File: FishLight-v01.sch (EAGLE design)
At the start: 214 parts, among them Q1 RK7002BSOT23-3, Q10 RK7002BSOT23-3, Q11 RK7002BSOT23-3, Q12 RK7002BSOT23-3, Q13 RK7002BSOT23-3, Q14 RK7002BSOT23-3, Q15 RK7002BSOT23-3, Q2 RK7002BSOT23-3, Q3 RK7002BSOT23-3, Q4 RK7002BSOT23-3, Q5 RK7002BSOT23-3, Q6 RK7002BSOT23-3, Q7 RK7002BSOT23-3, Q8 RK7002BSOT23-3, Q9 RK7002BSOT23-3, U1 SPARK_CORECORE, U10 AD5248MSOP-10, U11 INA219SOT23-8, U12 INA219SOT23-8, U13 INA219SOT23-8, U14 INA219SOT23-8, U15 INA219SOT23-8, U16 MIC29300D2PAK-3, U17 L7805D2PAK-2, U2 DS3231MSOIC-8, U22 AD5248MSOP-10, U23 CAT4101TO-263, U24 CAT4101TO-263, U25 CAT4101TO-263, U26 INA219SOT23-8, U27 INA219SOT23-8, U28 INA219SOT23-8, U29 CD74HC4067SSOP24, U3 CAT4101TO-263, U30 CD74HC4067SSOP24, U31 RELAY-SOLIDSTATEPTH, U32 RELAY-SOLIDSTATEPTH, U33 RELAY-SOLIDSTATEPTH, U34 NC7SZ373TSSOP-6, U35 NC7SZ373TSSOP-6, U36 NC7SZ373TSSOP-6, U37 NC7SZ373TSSOP-6, U38 NC7SZ373TSSOP-6, U39 NC7SZ373TSSOP-6, U4 CAT4101TO-263, U40 NC7SZ373TSSOP-6, U41 NC7SZ373TSSOP-6, U42 NC7SZ373TSSOP-6, U43 NC7SZ373TSSOP-6, U44 NC7SZ373TSSOP-6, U45 NC7SZ373TSSOP-6, U46 NC7SZ373TSSOP-6, U47 NC7SZ373TSSOP-6, U48 NC7SZ373TSSOP-6, U5 CAT4101TO-263, U6 CAT4101TO-263, U7 CAT4101TO-263, U8 AD5248MSOP-10, U9 AD5248MSOP-10

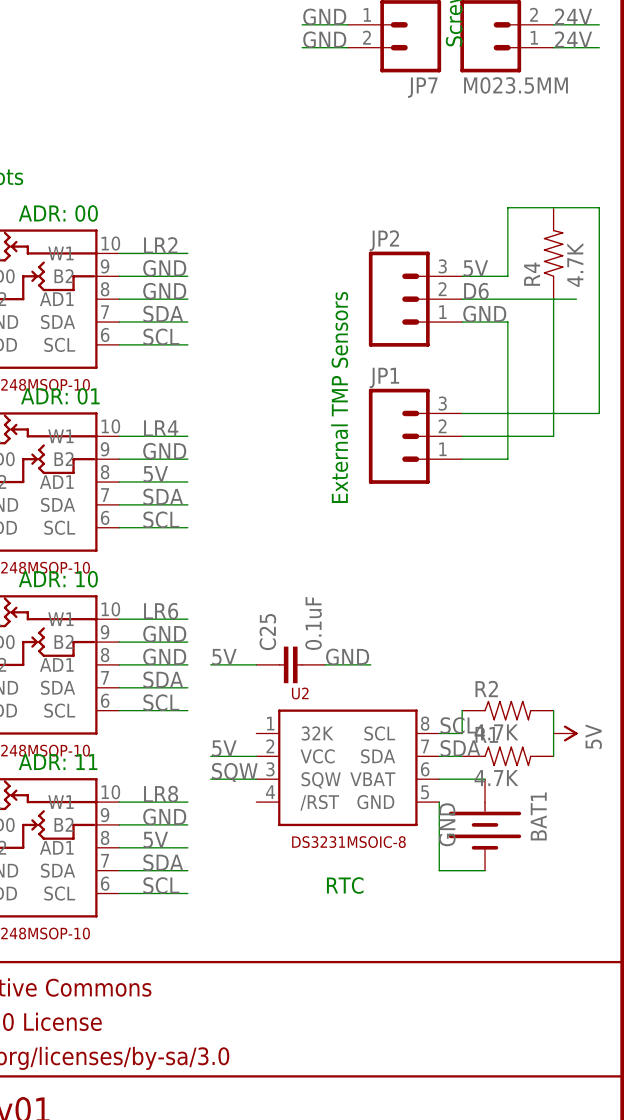
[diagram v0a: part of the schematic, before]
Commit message: FishLight_PCB: Routed power lines and sized them right
Moved a few things around and then routed the power lines for the
12V and 24V lines.  Also sized them appropriately for their max
current of about 7A and 15A respectively.
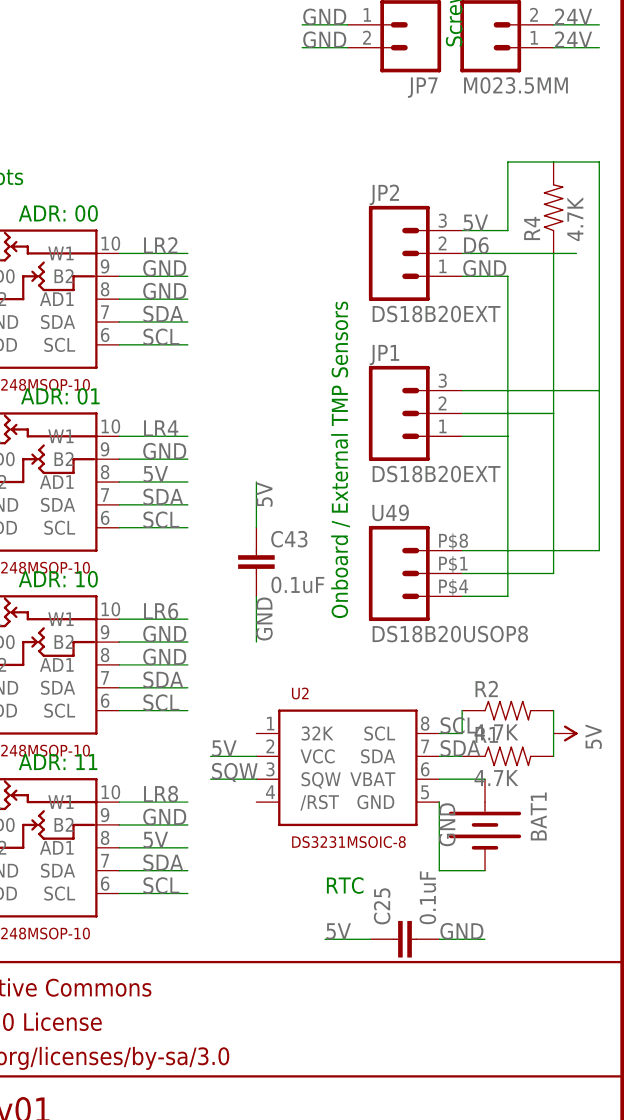
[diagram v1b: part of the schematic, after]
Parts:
- added C43: 0.1uF, SparkFun-Capacitors:0.1UF-25V(+80/-20%)(0603)
- added U49: DS18B20USOP8, Mikes-Stuff:DS18B20USOP8
- JP1, JP2: value (none) -> DS18B20EXT; device Mikes-Stuff:M03POLAR -> Mikes-Stuff:DS18B20EXT
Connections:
- net 5V: now also C43.1, JP1.VDD, JP2.VDD, U49.VDD; no longer JP1.3, JP2.3
- net D6: now also JP1.DQ, JP2.DQ, U49.DQ; no longer JP1.2, JP2.2
- net GND: now also C43.2, JP1.GND, JP2.GND, U49.GND; no longer JP1.1, JP2.1
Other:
- note added: "Onboard / External TMP Sensors"
- note removed: "External TMP Sensors"
- moved on the sheet: C25, JP1, JP2, R4
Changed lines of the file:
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@@
 <part name="C6" library="SparkFun-Capacitors" deviceset="0.1UF-100V-10%(0603)" device="" value="0.1uF"/>
 <part name="C12" library="SparkFun-Capacitors" deviceset="CAP" device="0603-CAP" value="0.33uF"/>
-<part name="JP2" library="Mikes-Stuff" deviceset="M03" device="POLAR"/>
+<part name="JP2" library="Mikes-Stuff" deviceset="DS18B20" device="EXT"/>
 <part name="JP9" library="Mikes-Stuff" deviceset="M03" device="SCREW"/>
 <part name="JP10" library="Mikes-Stuff" deviceset="M03" device="SCREW"/>
@@
 <part name="R59" library="SparkFun-Resistors" deviceset="RESISTOR" device="0603-RES" value="560"/>
 <part name="R60" library="SparkFun-Resistors" deviceset="RESISTOR" device="0603-RES" value="560"/>
-<part name="JP1" library="Mikes-Stuff" deviceset="M03" device="POLAR"/>
+<part name="JP1" library="Mikes-Stuff" deviceset="DS18B20" device="EXT"/>
+<part name="U49" library="Mikes-Stuff" deviceset="DS18B20" device="USOP8"/>
+<part name="C43" library="SparkFun-Capacitors" deviceset="0.1UF-25V(+80/-20%)(0603)" device="" value="0.1uF"/>
 </parts>
 <sheets>
@@
 <text x="129.54" y="182.88" size="1.778" layer="91">WW</text>
 <text x="162.56" y="182.88" size="1.778" layer="91">BL</text>
-<text x="218.44" y="86.36" size="1.778" layer="91" rot="R90">External TMP Sensors</text>
+<text x="218.44" y="73.66" size="1.778" layer="91" rot="R90">Onboard / External TMP Sensors</text>
 <text x="231.14" y="137.16" size="1.778" layer="91" rot="R90">Screw Terminals</text>
 <text x="91.44" y="119.38" size="1.778" layer="91">I-sense</text>
@@
 <instance part="C6" gate="G$1" x="33.02" y="10.16"/>
 <instance part="C12" gate="G$1" x="7.62" y="10.16"/>
-<instance part="JP2" gate="G$1" x="223.52" y="109.22"/>
+<instance part="JP2" gate="G$1" x="223.52" y="114.3"/>
 <instance part="JP9" gate="G$1" x="233.68" y="177.8"/>
 <instance part="JP10" gate="G$1" x="233.68" y="165.1"/>
@@
 <instance part="C15" gate="G$1" x="73.66" y="10.16"/>
 <instance part="U1" gate="G$1" x="25.4" y="152.4"/>
-<instance part="R4" gate="G$1" x="241.3" y="114.3" rot="R90"/>
+<instance part="R4" gate="G$1" x="241.3" y="119.38" rot="R90"/>
 <instance part="JP18" gate="G$1" x="5.08" y="111.76"/>
 <instance part="R6" gate="G$1" x="106.68" y="114.3" rot="R90"/>
@@
 <instance part="U2" gate="G$1" x="218.44" y="58.42"/>
 <instance part="BAT1" gate="G$1" x="233.68" y="50.8" rot="R270"/>
-<instance part="C25" gate="G$1" x="213.36" y="68.58" rot="R90"/>
+<instance part="C25" gate="G$1" x="226.06" y="38.1" rot="R90"/>
 <instance part="JP17" gate="G$1" x="38.1" y="-144.78"/>
 <instance part="JP19" gate="G$1" x="30.48" y="-142.24" rot="R180"/>
@@
 <instance part="R59" gate="G$1" x="25.4" y="76.2" rot="R90"/>
 <instance part="R60" gate="G$1" x="25.4" y="60.96" rot="R90"/>
-<instance part="JP1" gate="G$1" x="223.52" y="93.98"/>
+<instance part="JP1" gate="G$1" x="223.52" y="96.52"/>
+<instance part="U49" gate="G$1" x="223.52" y="78.74"/>
+<instance part="C43" gate="G$1" x="208.28" y="78.74"/>
 </instances>
 <busses>
@@
 </segment>
 <segment>
-<pinref part="JP2" gate="G$1" pin="1"/>
-<wire x1="231.14" y1="106.68" x2="236.22" y2="106.68" width="0.2032" layer="91"/>
-<label x="231.14" y="106.68" size="1.778" layer="95"/>
-<wire x1="236.22" y1="106.68" x2="236.22" y2="91.44" width="0.2032" layer="91"/>
-<pinref part="JP1" gate="G$1" pin="1"/>
-<wire x1="236.22" y1="91.44" x2="231.14" y2="91.44" width="0.2032" layer="91"/>
+<pinref part="JP2" gate="G$1" pin="GND"/>
+<wire x1="231.14" y1="111.76" x2="236.22" y2="111.76" width="0.2032" layer="91"/>
+<label x="231.14" y="111.76" size="1.778" layer="95"/>
+<wire x1="236.22" y1="111.76" x2="236.22" y2="93.98" width="0.2032" layer="91"/>
+<pinref part="JP1" gate="G$1" pin="GND"/>
+<wire x1="236.22" y1="93.98" x2="231.14" y2="93.98" width="0.2032" layer="91"/>
+<wire x1="236.22" y1="93.98" x2="236.22" y2="76.2" width="0.2032" layer="91"/>
+<pinref part="U49" gate="G$1" pin="GND"/>
+<wire x1="236.22" y1="76.2" x2="231.14" y2="76.2" width="0.2032" layer="91"/>
 </segment>
 <segment>
@@
 <segment>
 <pinref part="C25" gate="G$1" pin="2"/>
-<wire x1="215.9" y1="68.58" x2="220.98" y2="68.58" width="0.2032" layer="91"/>
-<label x="215.9" y="68.58" size="1.778" layer="95"/>
+<wire x1="228.6" y1="38.1" x2="233.68" y2="38.1" width="0.2032" layer="91"/>
+<label x="228.6" y="38.1" size="1.778" layer="95"/>
 </segment>
 <segment>
@@
 <wire x1="22.86" y1="83.82" x2="17.78" y2="83.82" width="0.2032" layer="91"/>
 </segment>
+<segment>
+<pinref part="C43" gate="G$1" pin="2"/>
+<wire x1="208.28" y1="76.2" x2="208.28" y2="71.12" width="0.2032" layer="91"/>
+<label x="208.28" y="76.2" size="1.778" layer="95" rot="R270"/>
+</segment>
 </net>
 <net name="5V" class="0">
@@
 </segment>
 <segment>
-<pinref part="JP2" gate="G$1" pin="3"/>
-<wire x1="231.14" y1="111.76" x2="236.22" y2="111.76" width="0.2032" layer="91"/>
-<label x="231.14" y="111.76" size="1.778" layer="95"/>
-<wire x1="236.22" y1="111.76" x2="236.22" y2="119.38" width="0.2032" layer="91"/>
+<pinref part="JP2" gate="G$1" pin="VDD"/>
+<wire x1="231.14" y1="116.84" x2="236.22" y2="116.84" width="0.2032" layer="91"/>
+<label x="231.14" y="116.84" size="1.778" layer="95"/>
+<wire x1="236.22" y1="116.84" x2="236.22" y2="124.46" width="0.2032" layer="91"/>
 <pinref part="R4" gate="G$1" pin="2"/>
-<wire x1="236.22" y1="119.38" x2="241.3" y2="119.38" width="0.2032" layer="91"/>
-<pinref part="JP1" gate="G$1" pin="3"/>
-<wire x1="231.14" y1="96.52" x2="246.38" y2="96.52" width="0.2032" layer="91"/>
-<wire x1="246.38" y1="96.52" x2="246.38" y2="119.38" width="0.2032" layer="91"/>
-<wire x1="246.38" y1="119.38" x2="241.3" y2="119.38" width="0.2032" layer="91"/>
+<wire x1="236.22" y1="124.46" x2="241.3" y2="124.46" width="0.2032" layer="91"/>
+<pinref part="JP1" gate="G$1" pin="VDD"/>
+<wire x1="231.14" y1="99.06" x2="246.38" y2="99.06" width="0.2032" layer="91"/>
+<wire x1="246.38" y1="99.06" x2="246.38" y2="124.46" width="0.2032" layer="91"/>
+<wire x1="246.38" y1="124.46" x2="241.3" y2="124.46" width="0.2032" layer="91"/>
+<pinref part="U49" gate="G$1" pin="VDD"/>
+<wire x1="231.14" y1="81.28" x2="246.38" y2="81.28" width="0.2032" layer="91"/>
+<wire x1="246.38" y1="81.28" x2="246.38" y2="99.06" width="0.2032" layer="91"/>
 </segment>
 <segment>
@@
 <segment>
 <pinref part="C25" gate="G$1" pin="1"/>
-<wire x1="208.28" y1="68.58" x2="203.2" y2="68.58" width="0.2032" layer="91"/>
-<label x="203.2" y="68.58" size="1.778" layer="95"/>
+<wire x1="220.98" y1="38.1" x2="215.9" y2="38.1" width="0.2032" layer="91"/>
+<label x="215.9" y="38.1" size="1.778" layer="95"/>
 </segment>
 <segment>
@@
 <label x="30.48" y="81.28" size="1.778" layer="95"/>
 </segment>
+<segment>
+<pinref part="C43" gate="G$1" pin="1"/>
+<wire x1="208.28" y1="83.82" x2="208.28" y2="88.9" width="0.2032" layer="91"/>
+<label x="208.28" y="88.9" size="1.778" layer="95" rot="R270"/>
+</segment>
 </net>
 <net name="SQW" class="0">
@@
 <segment>
 <pinref part="R4" gate="G$1" pin="1"/>
-<pinref part="JP2" gate="G$1" pin="2"/>
-<wire x1="241.3" y1="109.22" x2="231.14" y2="109.22" width="0.2032" layer="91"/>
-<label x="231.14" y="109.22" size="1.778" layer="95"/>
-<pinref part="JP1" gate="G$1" pin="2"/>
-<wire x1="241.3" y1="109.22" x2="241.3" y2="93.98" width="0.2032" layer="91"/>
-<wire x1="241.3" y1="93.98" x2="231.14" y2="93.98" width="0.2032" layer="91"/>
-<wire x1="241.3" y1="109.22" x2="243.84" y2="109.22" width="0.2032" layer="91"/>
+<pinref part="JP2" gate="G$1" pin="DQ"/>
+<wire x1="241.3" y1="114.3" x2="231.14" y2="114.3" width="0.2032" layer="91"/>
+<label x="231.14" y="114.3" size="1.778" layer="95"/>
+<pinref part="JP1" gate="G$1" pin="DQ"/>
+<wire x1="241.3" y1="114.3" x2="241.3" y2="96.52" width="0.2032" layer="91"/>
+<wire x1="241.3" y1="96.52" x2="231.14" y2="96.52" width="0.2032" layer="91"/>
+<wire x1="241.3" y1="114.3" x2="243.84" y2="114.3" width="0.2032" layer="91"/>
+<pinref part="U49" gate="G$1" pin="DQ"/>
+<wire x1="231.14" y1="78.74" x2="241.3" y2="78.74" width="0.2032" layer="91"/>
+<wire x1="241.3" y1="78.74" x2="241.3" y2="96.52" width="0.2032" layer="91"/>
 </segment>
 </net>
